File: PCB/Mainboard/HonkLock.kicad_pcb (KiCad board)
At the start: 2 copper layers, 41 x 47 mm, 15 parts, among them J1 Conn_01x03_Pin, J5 Conn_01x02_Pin, U2 ESP32-S3-SUPERMINI

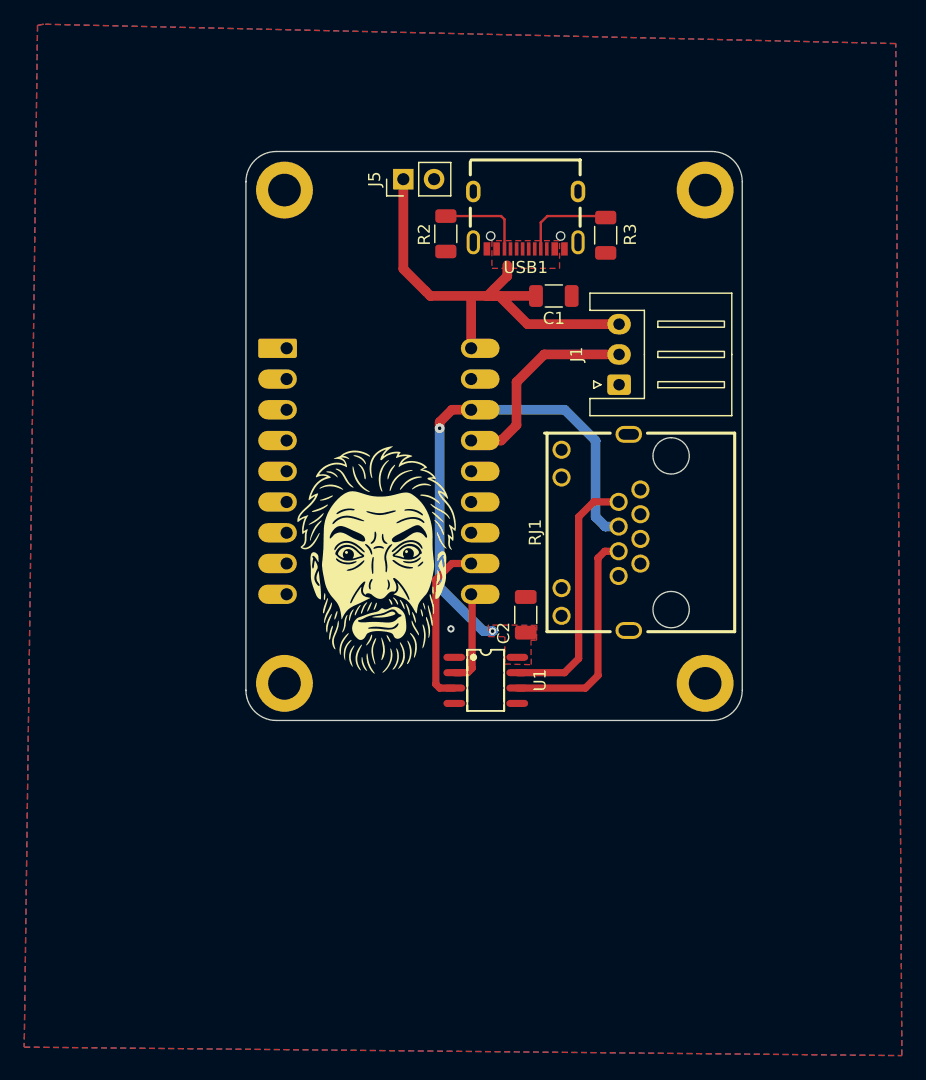
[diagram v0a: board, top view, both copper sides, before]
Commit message: Mainboard ready for mfg
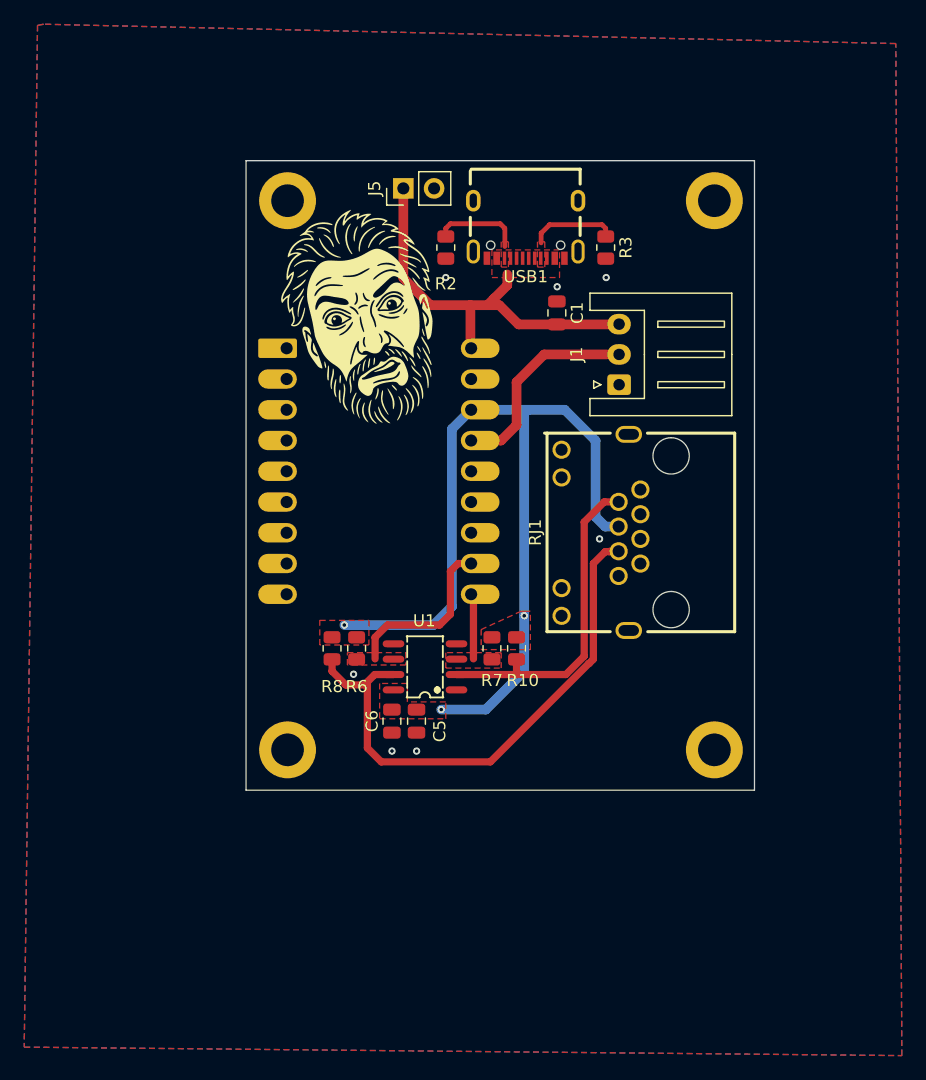
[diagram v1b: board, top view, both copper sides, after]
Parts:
- removed C2: 0.1uF, Capacitor_SMD:C_1206_3216Metric
- added C5: 0.1uF, Capacitor_SMD:C_0805_2012Metric, F.Cu at (129.4, 82.9)
- added C6: 1uF, Capacitor_SMD:C_0805_2012Metric, F.Cu at (127.4, 82.9)
- added R10: 10k, Resistor_SMD:R_0805_2012Metric, F.Cu at (137.7, 76.9)
- added R6: 33k, Resistor_SMD:R_0805_2012Metric, F.Cu at (124.5, 76.9)
- added R7: 33k, Resistor_SMD:R_0805_2012Metric, F.Cu at (135.6, 76.9)
- added R8: 10k, Resistor_SMD:R_0805_2012Metric, F.Cu at (122.4, 76.9)
- C1: footprint Capacitor_SMD:C_1206_3216Metric -> Capacitor_SMD:C_0805_2012Metric
- R2, R3: footprint Resistor_SMD:R_1206_3216Metric -> Resistor_SMD:R_0805_2012Metric
- moved REF** 5.54 mm to (154.0, 85.2)
- moved REF** 5.50 mm to (118.8, 85.2)
- moved U1 5.14 mm to (130.1, 78.4), turned to 90 degrees
- moved C1 1.42 mm to (141.0, 49.1), turned to -90 degrees
- moved REF** 1.16 mm to (154.0, 39.9)
- moved R2 1.14 mm to (131.8, 43.7)
- moved R3 1.02 mm to (145.0, 43.7)
- moved REF** 0.91 mm to (118.8, 39.9)
- moved J5 0.76 mm to (128.3, 38.9)
- moved USB1 0.76 mm to (138.4, 42.3)
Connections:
- RJ1 pad 2: Net-(U1-LY) -> BusSDA
- RJ1 pad 6: Net-(U1-SY) -> BusSCL
- U1 pad 2: Sensor1SCK -> BusSDA
- U1 pad 3: Sensor1SDA -> MCUSDA
- U1 pad 6: Net-(U1-SY) -> MCUSCL
- U1 pad 7: Net-(U1-LY) -> BusSCL
- U2 pad 8: Sensor1SCK -> MCUSDA
- U2 pad 9: Sensor1SDA -> MCUSCL
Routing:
- net BusSCL: track 0.00 -> 45.3 mm
- net 3v3: track 42.5 -> 76.1 mm, vias 2 -> 3
- net BusSDA: track 0.00 -> 27.0 mm
- net Net-(U1-LY): track 21.1 -> 0.00 mm
- net Net-(U1-SY): track 18.7 -> 0.00 mm
- net MCUSCL: track 0.00 -> 14.5 mm
- net Sensor1SDA: track 13.8 -> 0.00 mm
- net Sensor1SCK: track 7.77 -> 0.00 mm
- net MCUSDA: track 0.00 -> 5.41 mm
- net VDD: track 37.7 -> 33.6 mm
- net GND: vias 1 -> 7
- added copper zone on F.Cu, net MCUSCL
- added copper zone on F.Cu, net MCUSDA
- added copper zone on F.Cu, net Net-(USB1-CC1)
- added copper zone on F.Cu, net Net-(USB1-CC2)
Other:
- board size 41 x 47 mm -> 42 x 52 mm
